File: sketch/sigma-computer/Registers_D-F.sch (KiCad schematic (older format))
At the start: 12 parts

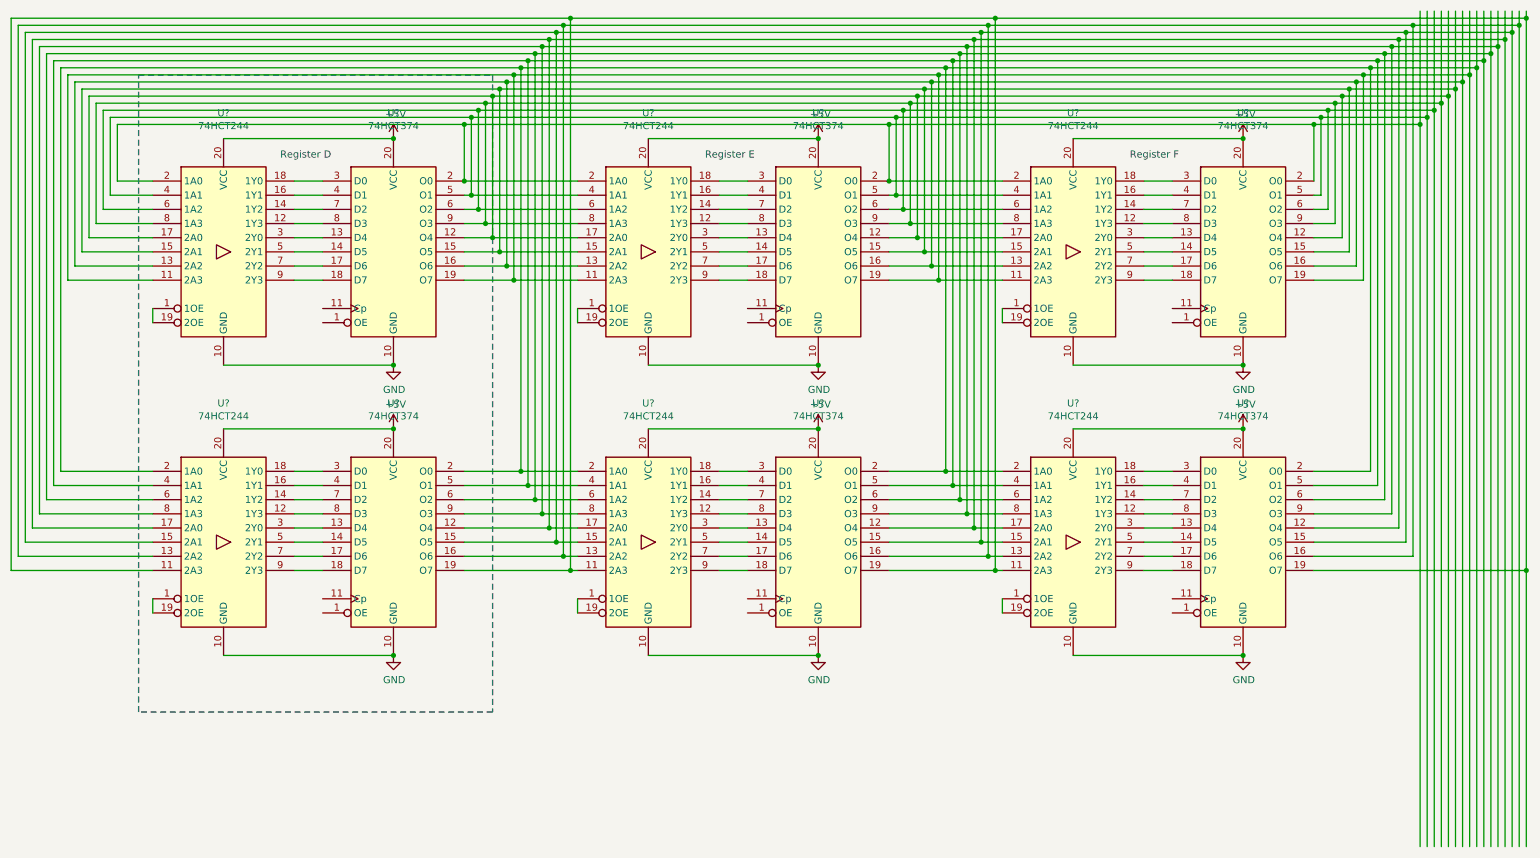
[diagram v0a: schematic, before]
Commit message: Changes in the schematic
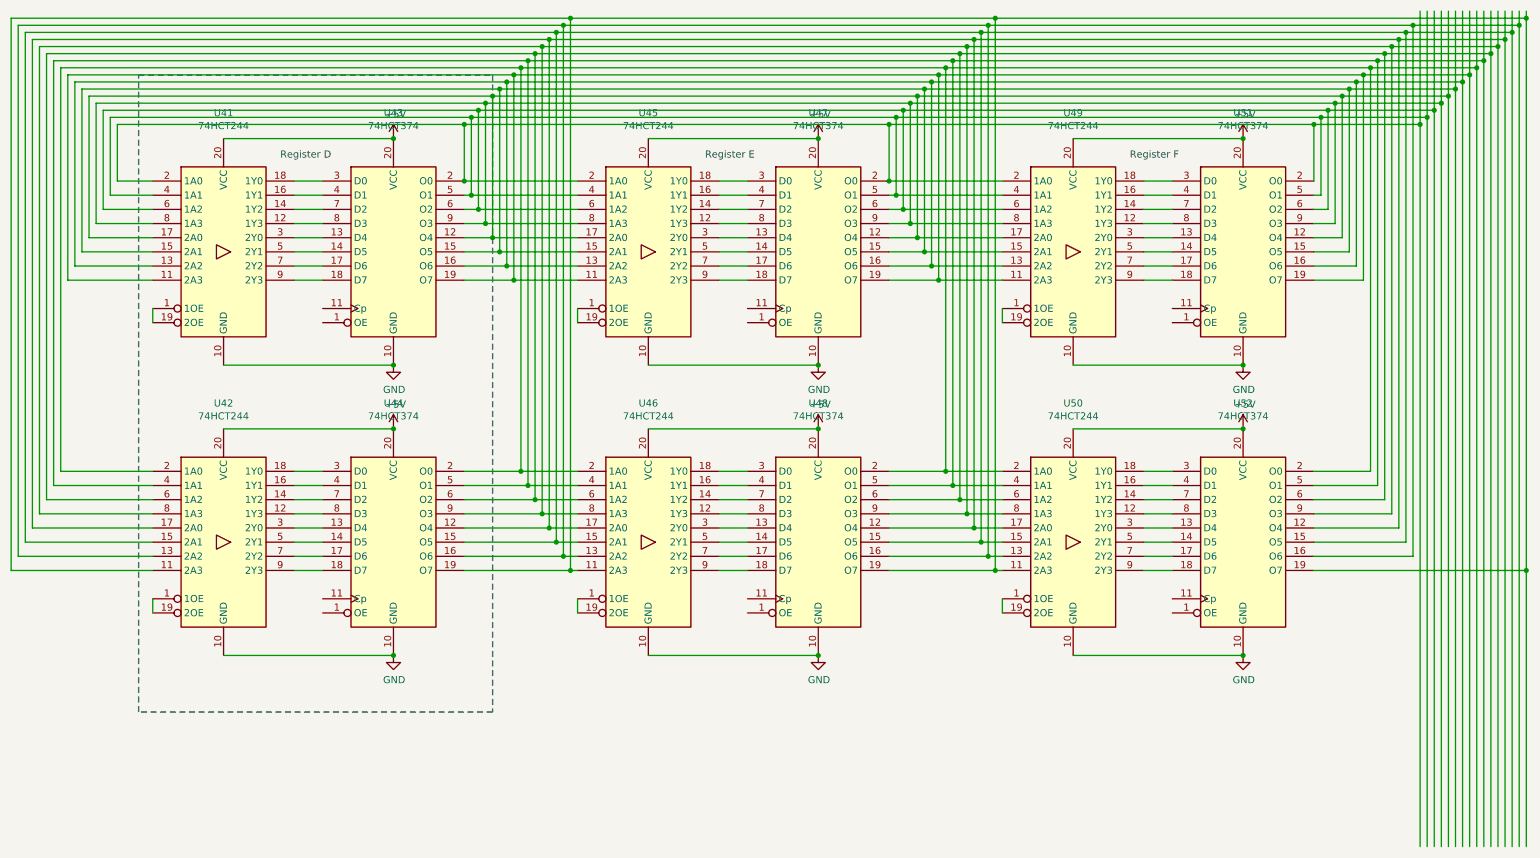
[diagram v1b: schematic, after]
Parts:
- removed U? (x3): 74HCT374, symbol 74xx:74HCT374
- removed U? (x3): 74HCT244, symbol 74xx:74HCT244
- added U41, U49, U50: 74HCT244, symbol 74xx:74HCT244
- added U43, U51, U52: 74HCT374, symbol 74xx:74HCT374
- gave numbers to parts that had none: 6
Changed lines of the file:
@@
 P 3200 5050
 AR Path="/5D32333B/5D29A080" Ref="#PWR?"  Part="1"
-AR Path="/5D28F068/5D29A080" Ref="#PWR?"  Part="1"
-F 0 "#PWR?" H 3200 4800 50  0001 C CNN
+AR Path="/5D28F068/5D29A080" Ref="#PWR0137"  Part="1"
+F 0 "#PWR0137" H 3200 4800 50  0001 C CNN
 F 1 "GND" H 3205 4877 50  0000 C CNN
 F 2 "" H 3200 5050 50  0001 C CNN
@@
 P 3200 3450
 AR Path="/5D32333B/5D29A079" Ref="#PWR?"  Part="1"
-AR Path="/5D28F068/5D29A079" Ref="#PWR?"  Part="1"
-F 0 "#PWR?" H 3200 3300 50  0001 C CNN
+AR Path="/5D28F068/5D29A079" Ref="#PWR0138"  Part="1"
+F 0 "#PWR0138" H 3200 3300 50  0001 C CNN
 F 1 "+5V" H 3215 3623 50  0000 C CNN
 F 2 "" H 3200 3450 50  0001 C CNN
@@
 P 2000 4250
 AR Path="/5D32333B/5D29A068" Ref="U?"  Part="1"
-AR Path="/5D28F068/5D29A068" Ref="U?"  Part="1"
-F 0 "U?" H 2000 5231 50  0000 C CNN
+AR Path="/5D28F068/5D29A068" Ref="U42"  Part="1"
+F 0 "U42" H 2000 5231 50  0000 C CNN
 F 1 "74HCT244" H 2000 5140 50  0000 C CNN
 F 2 "" H 2000 4250 50  0001 C CNN
@@
 P 3200 4250
 AR Path="/5D32333B/5D29A062" Ref="U?"  Part="1"
-AR Path="/5D28F068/5D29A062" Ref="U?"  Part="1"
-F 0 "U?" H 3200 5231 50  0000 C CNN
+AR Path="/5D28F068/5D29A062" Ref="U44"  Part="1"
+F 0 "U44" H 3200 5231 50  0000 C CNN
 F 1 "74HCT374" H 3200 5140 50  0000 C CNN
 F 2 "" H 3200 4250 50  0001 C CNN
@@
 P 3200 3000
 AR Path="/5D32333B/5D292607" Ref="#PWR?"  Part="1"
-AR Path="/5D28F068/5D292607" Ref="#PWR?"  Part="1"
-F 0 "#PWR?" H 3200 2750 50  0001 C CNN
+AR Path="/5D28F068/5D292607" Ref="#PWR0139"  Part="1"
+F 0 "#PWR0139" H 3200 2750 50  0001 C CNN
 F 1 "GND" H 3205 2827 50  0000 C CNN
 F 2 "" H 3200 3000 50  0001 C CNN
@@
 $Comp
 L power:+5V #PWR?
-U 1 1 5D291F0D
+U 1 1 5D5C57A4
 P 3200 1400
-AR Path="/5D32333B/5D291F0D" Ref="#PWR?"  Part="1"
-AR Path="/5D28F068/5D291F0D" Ref="#PWR?"  Part="1"
-F 0 "#PWR?" H 3200 1250 50  0001 C CNN
+AR Path="/5D32333B/5D5C57A4" Ref="#PWR?"  Part="1"
+AR Path="/5D28F068/5D5C57A4" Ref="#PWR0140"  Part="1"
+F 0 "#PWR0140" H 3200 1250 50  0001 C CNN
 F 1 "+5V" H 3215 1573 50  0000 C CNN
 F 2 "" H 3200 1400 50  0001 C CNN
@@
 $Comp
 L 74xx:74HCT244 U?
-U 1 1 5D28CD6D
+U 1 1 5D5C57A3
 P 2000 2200
-AR Path="/5D32333B/5D28CD6D" Ref="U?"  Part="1"
-AR Path="/5D28F068/5D28CD6D" Ref="U?"  Part="1"
-F 0 "U?" H 2000 3181 50  0000 C CNN
+AR Path="/5D32333B/5D5C57A3" Ref="U?"  Part="1"
+AR Path="/5D28F068/5D5C57A3" Ref="U41"  Part="1"
+F 0 "U41" H 2000 3181 50  0000 C CNN
 F 1 "74HCT244" H 2000 3090 50  0000 C CNN
 F 2 "" H 2000 2200 50  0001 C CNN
@@
 $Comp
 L 74xx:74HCT374 U?
-U 1 1 5D28A3E8
+U 1 1 5D5C57A2
 P 3200 2200
-AR Path="/5D32333B/5D28A3E8" Ref="U?"  Part="1"
-AR Path="/5D28F068/5D28A3E8" Ref="U?"  Part="1"
-F 0 "U?" H 3200 3181 50  0000 C CNN
+AR Path="/5D32333B/5D5C57A2" Ref="U?"  Part="1"
+AR Path="/5D28F068/5D5C57A2" Ref="U43"  Part="1"
+F 0 "U43" H 3200 3181 50  0000 C CNN
 F 1 "74HCT374" H 3200 3090 50  0000 C CNN
 F 2 "" H 3200 2200 50  0001 C CNN
@@
 P 6200 5050
 AR Path="/5D32333B/5D36E9E8" Ref="#PWR?"  Part="1"
-AR Path="/5D28F068/5D36E9E8" Ref="#PWR?"  Part="1"
-F 0 "#PWR?" H 6200 4800 50  0001 C CNN
+AR Path="/5D28F068/5D36E9E8" Ref="#PWR0141"  Part="1"
+F 0 "#PWR0141" H 6200 4800 50  0001 C CNN
 F 1 "GND" H 6205 4877 50  0000 C CNN
 F 2 "" H 6200 5050 50  0001 C CNN
@@
 P 6200 3450
 AR Path="/5D32333B/5D36E9F3" Ref="#PWR?"  Part="1"
-AR Path="/5D28F068/5D36E9F3" Ref="#PWR?"  Part="1"
-F 0 "#PWR?" H 6200 3300 50  0001 C CNN
+AR Path="/5D28F068/5D36E9F3" Ref="#PWR0142"  Part="1"
+F 0 "#PWR0142" H 6200 3300 50  0001 C CNN
 F 1 "+5V" H 6215 3623 50  0000 C CNN
 F 2 "" H 6200 3450 50  0001 C CNN
@@
 P 5000 4250
 AR Path="/5D32333B/5D36EA02" Ref="U?"  Part="1"
-AR Path="/5D28F068/5D36EA02" Ref="U?"  Part="1"
-F 0 "U?" H 5000 5231 50  0000 C CNN
+AR Path="/5D28F068/5D36EA02" Ref="U46"  Part="1"
+F 0 "U46" H 5000 5231 50  0000 C CNN
 F 1 "74HCT244" H 5000 5140 50  0000 C CNN
 F 2 "" H 5000 4250 50  0001 C CNN
@@
 P 6200 4250
 AR Path="/5D32333B/5D36EA08" Ref="U?"  Part="1"
-AR Path="/5D28F068/5D36EA08" Ref="U?"  Part="1"
-F 0 "U?" H 6200 5231 50  0000 C CNN
+AR Path="/5D28F068/5D36EA08" Ref="U48"  Part="1"
+F 0 "U48" H 6200 5231 50  0000 C CNN
 F 1 "74HCT374" H 6200 5140 50  0000 C CNN
 F 2 "" H 6200 4250 50  0001 C CNN
@@
 P 6200 3000
 AR Path="/5D32333B/5D36EA0F" Ref="#PWR?"  Part="1"
-AR Path="/5D28F068/5D36EA0F" Ref="#PWR?"  Part="1"
-F 0 "#PWR?" H 6200 2750 50  0001 C CNN
+AR Path="/5D28F068/5D36EA0F" Ref="#PWR0143"  Part="1"
+F 0 "#PWR0143" H 6200 2750 50  0001 C CNN
 F 1 "GND" H 6205 2827 50  0000 C CNN
 F 2 "" H 6200 3000 50  0001 C CNN
@@
 P 6200 1400
 AR Path="/5D32333B/5D36EA16" Ref="#PWR?"  Part="1"
-AR Path="/5D28F068/5D36EA16" Ref="#PWR?"  Part="1"
-F 0 "#PWR?" H 6200 1250 50  0001 C CNN
+AR Path="/5D28F068/5D36EA16" Ref="#PWR0144"  Part="1"
+F 0 "#PWR0144" H 6200 1250 50  0001 C CNN
 F 1 "+5V" H 6215 1573 50  0000 C CNN
 F 2 "" H 6200 1400 50  0001 C CNN
@@
 P 5000 2200
 AR Path="/5D32333B/5D36EA26" Ref="U?"  Part="1"
-AR Path="/5D28F068/5D36EA26" Ref="U?"  Part="1"
-F 0 "U?" H 5000 3181 50  0000 C CNN
+AR Path="/5D28F068/5D36EA26" Ref="U45"  Part="1"
+F 0 "U45" H 5000 3181 50  0000 C CNN
 F 1 "74HCT244" H 5000 3090 50  0000 C CNN
 F 2 "" H 5000 2200 50  0001 C CNN
@@
 P 6200 2200
 AR Path="/5D32333B/5D36EA2C" Ref="U?"  Part="1"
-AR Path="/5D28F068/5D36EA2C" Ref="U?"  Part="1"
-F 0 "U?" H 6200 3181 50  0000 C CNN
+AR Path="/5D28F068/5D36EA2C" Ref="U47"  Part="1"
+F 0 "U47" H 6200 3181 50  0000 C CNN
 F 1 "74HCT374" H 6200 3090 50  0000 C CNN
 F 2 "" H 6200 2200 50  0001 C CNN
@@
 $Comp
 L 74xx:74HCT374 U?
-U 1 1 5D5D64F6
+U 1 1 5D5C57B9
 P 9200 2200
-AR Path="/5D32333B/5D5D64F6" Ref="U?"  Part="1"
-AR Path="/5D28F068/5D5D64F6" Ref="U?"  Part="1"
-F 0 "U?" H 9200 3181 50  0000 C CNN
+AR Path="/5D32333B/5D5C57B9" Ref="U?"  Part="1"
+AR Path="/5D28F068/5D5C57B9" Ref="U51"  Part="1"
+F 0 "U51" H 9200 3181 50  0000 C CNN
 F 1 "74HCT374" H 9200 3090 50  0000 C CNN
 F 2 "" H 9200 2200 50  0001 C CNN
@@
 $Comp
 L 74xx:74HCT244 U?
-U 1 1 5D5D64F0
+U 1 1 5D5C57B8
 P 8000 2200
-AR Path="/5D32333B/5D5D64F0" Ref="U?"  Part="1"
-AR Path="/5D28F068/5D5D64F0" Ref="U?"  Part="1"
-F 0 "U?" H 8000 3181 50  0000 C CNN
+AR Path="/5D32333B/5D5C57B8" Ref="U?"  Part="1"
+AR Path="/5D28F068/5D5C57B8" Ref="U49"  Part="1"
+F 0 "U49" H 8000 3181 50  0000 C CNN
 F 1 "74HCT244" H 8000 3090 50  0000 C CNN
 F 2 "" H 8000 2200 50  0001 C CNN
@@
 P 9200 1400
 AR Path="/5D32333B/5D5D64E0" Ref="#PWR?"  Part="1"
-AR Path="/5D28F068/5D5D64E0" Ref="#PWR?"  Part="1"
-F 0 "#PWR?" H 9200 1250 50  0001 C CNN
+AR Path="/5D28F068/5D5D64E0" Ref="#PWR0145"  Part="1"
+F 0 "#PWR0145" H 9200 1250 50  0001 C CNN
 F 1 "+5V" H 9215 1573 50  0000 C CNN
 F 2 "" H 9200 1400 50  0001 C CNN
@@
 $Comp
 L power:GND #PWR?
-U 1 1 5D5D64D9
+U 1 1 5D5C57B6
 P 9200 3000
-AR Path="/5D32333B/5D5D64D9" Ref="#PWR?"  Part="1"
-AR Path="/5D28F068/5D5D64D9" Ref="#PWR?"  Part="1"
-F 0 "#PWR?" H 9200 2750 50  0001 C CNN
+AR Path="/5D32333B/5D5C57B6" Ref="#PWR?"  Part="1"
+AR Path="/5D28F068/5D5C57B6" Ref="#PWR0146"  Part="1"
+F 0 "#PWR0146" H 9200 2750 50  0001 C CNN
 F 1 "GND" H 9205 2827 50  0000 C CNN
 F 2 "" H 9200 3000 50  0001 C CNN
@@
 $Comp
 L 74xx:74HCT374 U?
-U 1 1 5D5D64D2
+U 1 1 5D5C57B5
 P 9200 4250
-AR Path="/5D32333B/5D5D64D2" Ref="U?"  Part="1"
-AR Path="/5D28F068/5D5D64D2" Ref="U?"  Part="1"
-F 0 "U?" H 9200 5231 50  0000 C CNN
+AR Path="/5D32333B/5D5C57B5" Ref="U?"  Part="1"
+AR Path="/5D28F068/5D5C57B5" Ref="U52"  Part="1"
+F 0 "U52" H 9200 5231 50  0000 C CNN
 F 1 "74HCT374" H 9200 5140 50  0000 C CNN
 F 2 "" H 9200 4250 50  0001 C CNN
@@
 $Comp
 L 74xx:74HCT244 U?
-U 1 1 5D5D64CC
+U 1 1 5D5C57B4
 P 8000 4250
-AR Path="/5D32333B/5D5D64CC" Ref="U?"  Part="1"
-AR Path="/5D28F068/5D5D64CC" Ref="U?"  Part="1"
-F 0 "U?" H 8000 5231 50  0000 C CNN
+AR Path="/5D32333B/5D5C57B4" Ref="U?"  Part="1"
+AR Path="/5D28F068/5D5C57B4" Ref="U50"  Part="1"
+F 0 "U50" H 8000 5231 50  0000 C CNN
 F 1 "74HCT244" H 8000 5140 50  0000 C CNN
 F 2 "" H 8000 4250 50  0001 C CNN
@@
 P 9200 3450
 AR Path="/5D32333B/5D5D64BD" Ref="#PWR?"  Part="1"
-AR Path="/5D28F068/5D5D64BD" Ref="#PWR?"  Part="1"
-F 0 "#PWR?" H 9200 3300 50  0001 C CNN
+AR Path="/5D28F068/5D5D64BD" Ref="#PWR0147"  Part="1"
+F 0 "#PWR0147" H 9200 3300 50  0001 C CNN
 F 1 "+5V" H 9215 3623 50  0000 C CNN
 F 2 "" H 9200 3450 50  0001 C CNN
@@
 P 9200 5050
 AR Path="/5D32333B/5D5D64B3" Ref="#PWR?"  Part="1"
-AR Path="/5D28F068/5D5D64B3" Ref="#PWR?"  Part="1"
-F 0 "#PWR?" H 9200 4800 50  0001 C CNN
+AR Path="/5D28F068/5D5D64B3" Ref="#PWR0148"  Part="1"
+F 0 "#PWR0148" H 9200 4800 50  0001 C CNN
 F 1 "GND" H 9205 4877 50  0000 C CNN
 F 2 "" H 9200 5050 50  0001 C CNN
